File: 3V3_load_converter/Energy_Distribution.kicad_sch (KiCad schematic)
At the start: 23 parts, among them J10 532610271, J17 532610671, J18 532610271, J9 532610671, U17 NVTFS5116PLTAG, U18 NVTFS5116PLTAG, U19 INA199C3DCKR, U37 LMV321RIYLT, U39 NVTFS5116PLTAG, U40 NVTFS5116PLTAG

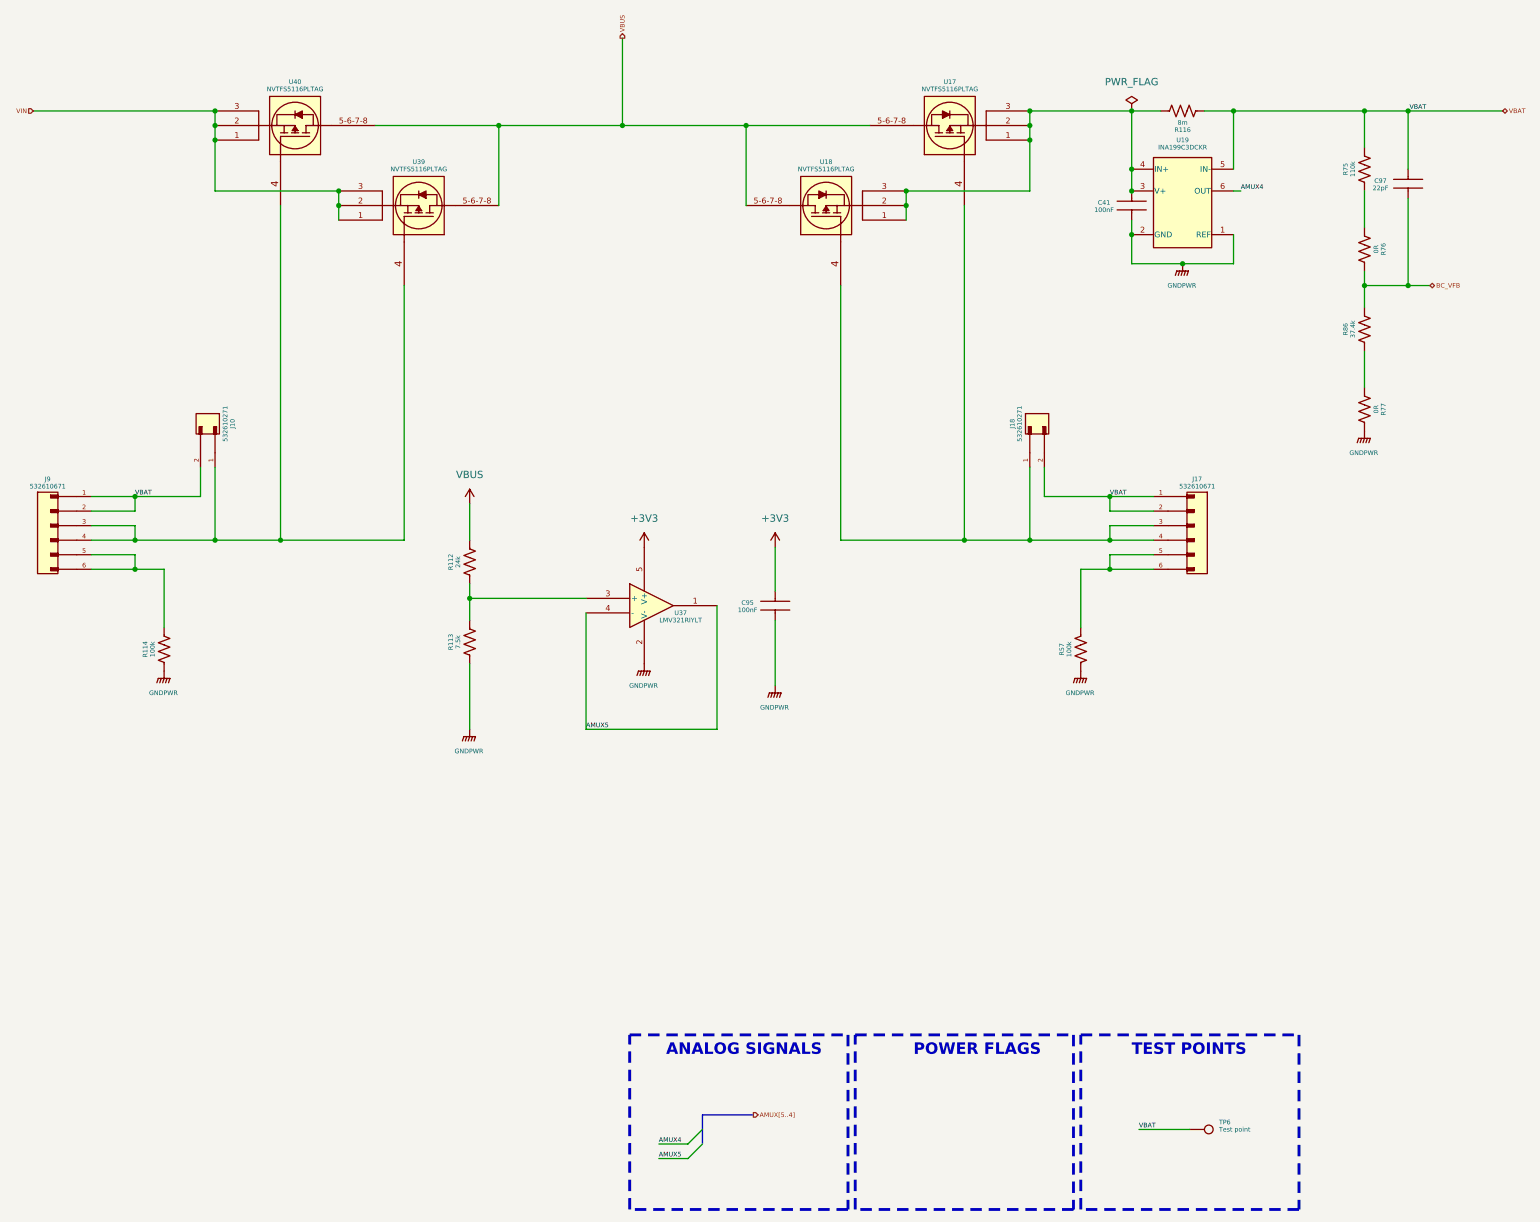
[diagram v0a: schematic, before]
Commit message: update
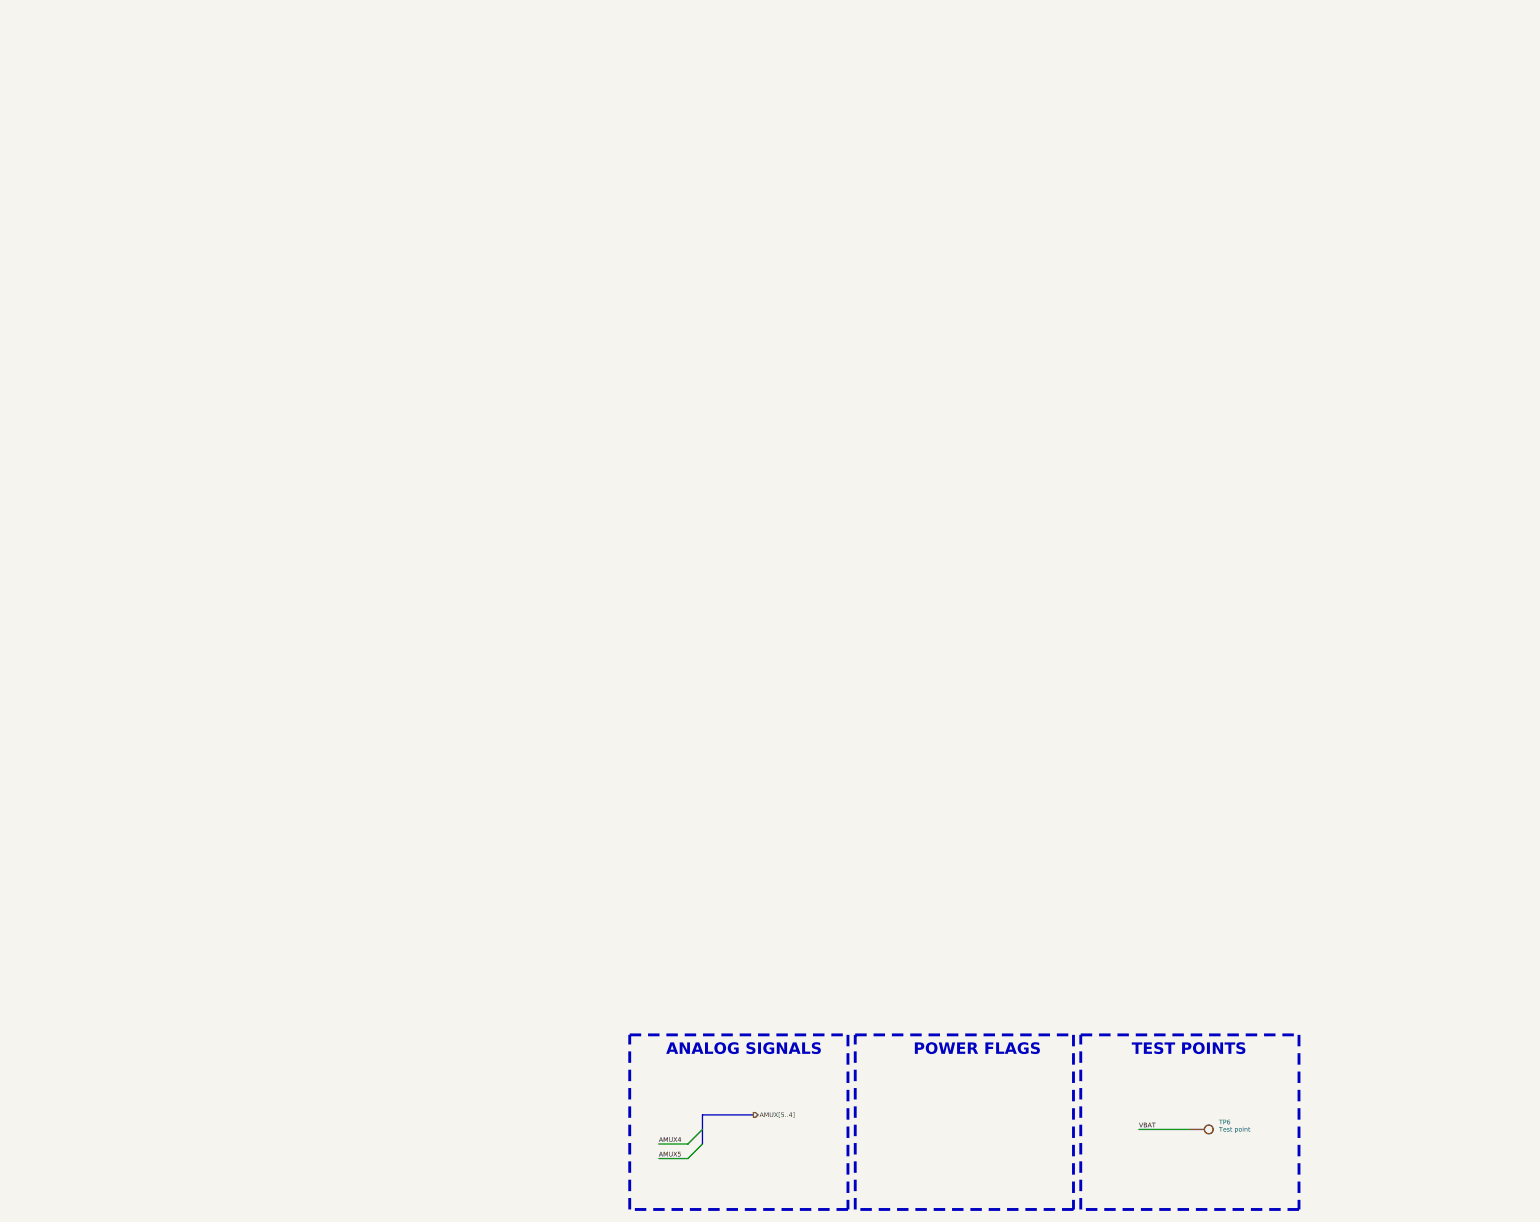
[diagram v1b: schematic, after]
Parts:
- removed C41, C95: 100nF, footprints:CAP0603, symbol C0603C104K5RACTU:C0603C104K5RACTU
- removed C97: 22pF, footprints:CAP0603, symbol C0603C220K5RACAUTO:C0603C220K5RACAUTO
- removed J10, J18: 532610271, footprints:532610271, symbol 532610271:532610271
- removed J17, J9: 532610671, footprints:532610671, symbol 532610671:532610671
- removed R112: 24k, footprints:RES0603, symbol CRCW060324K0FKEAHP:CRCW060324K0FKEAHP
- removed R113: 7.5k, footprints:RES0603, symbol CRCW06037K50FKEAHP:CRCW06037K50FKEAHP
- removed R114, R57: 100k, footprints:RES0603, symbol CRCW0603100KFKEAHP:CRCW0603100KFKEAHP
- removed R116: 8m, footprints:RES2010, symbol WSL20108L000FEA18:WSL20108L000FEA18
- removed R75: 110k, footprints:RES0603, symbol CRCW0603110KFKEAHP:CRCW0603110KFKEAHP
- removed R76, R77: 0R, footprints:RES0603, symbol CRCW06030000Z0EAHP:CRCW06030000Z0EAHP
- removed R86: 37.4k, footprints:RES0603, symbol CRCW060337K4FKEAHP:CRCW060337K4FKEAHP
- removed U17, U18, U39, U40: NVTFS5116PLTAG, footprints:NVTFS5116PLTAG, symbol NVTFS5116PLWFTAG:NVTFS5116PLTAG
- removed U19: INA199C3DCKR, footprints:INA199C3DCKR, symbol INA199C3DCKR:INA199C3DCKR
- removed U37: LMV321RIYLT, footprints:LMV321RIYLT, symbol LMV321RIYLT:LMV321RIYLT
